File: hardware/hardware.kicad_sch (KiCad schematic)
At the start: 14 parts, among them J1 AVR-ISP-6, U1 AMS1117-3.3, U2 ATmega88PA-A, U3 CH340C, U4 MPU-6050, Y1 Crystal

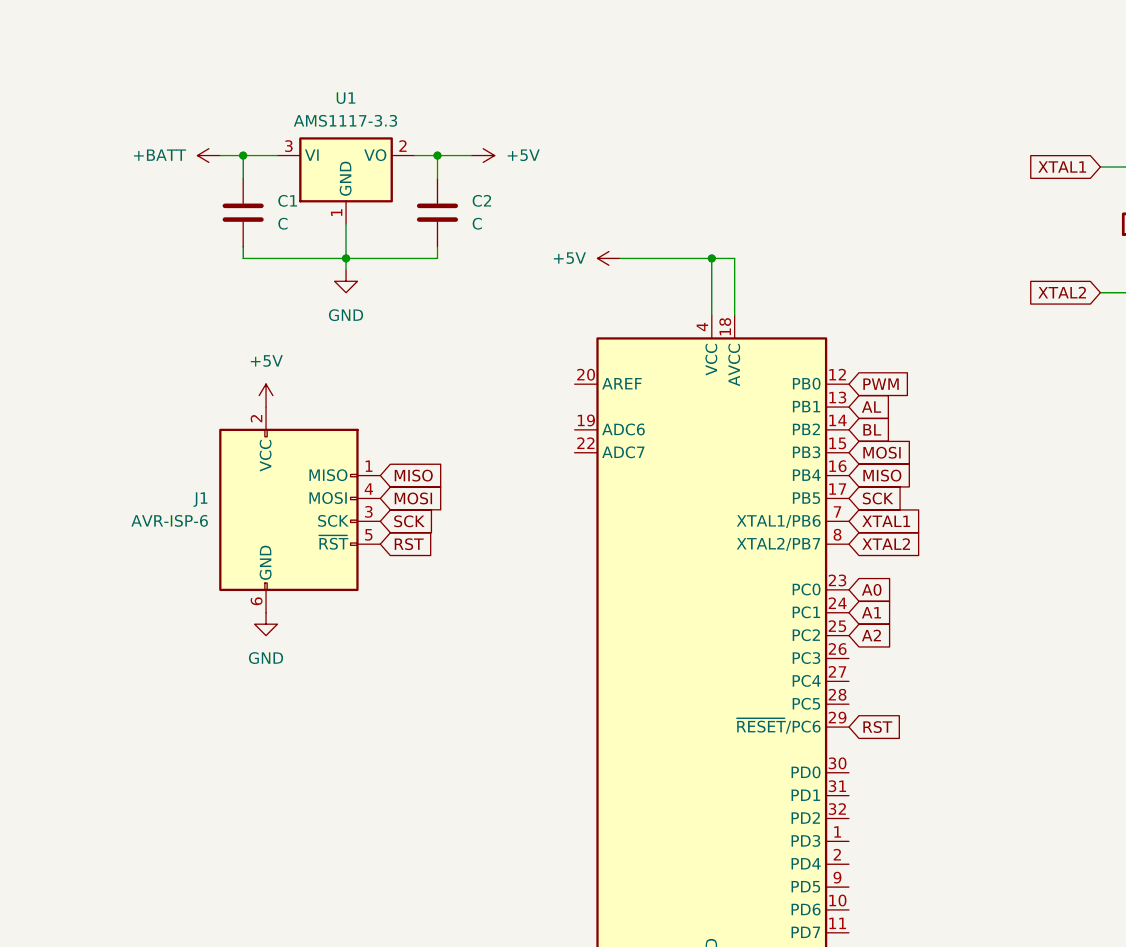
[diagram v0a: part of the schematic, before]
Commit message: up
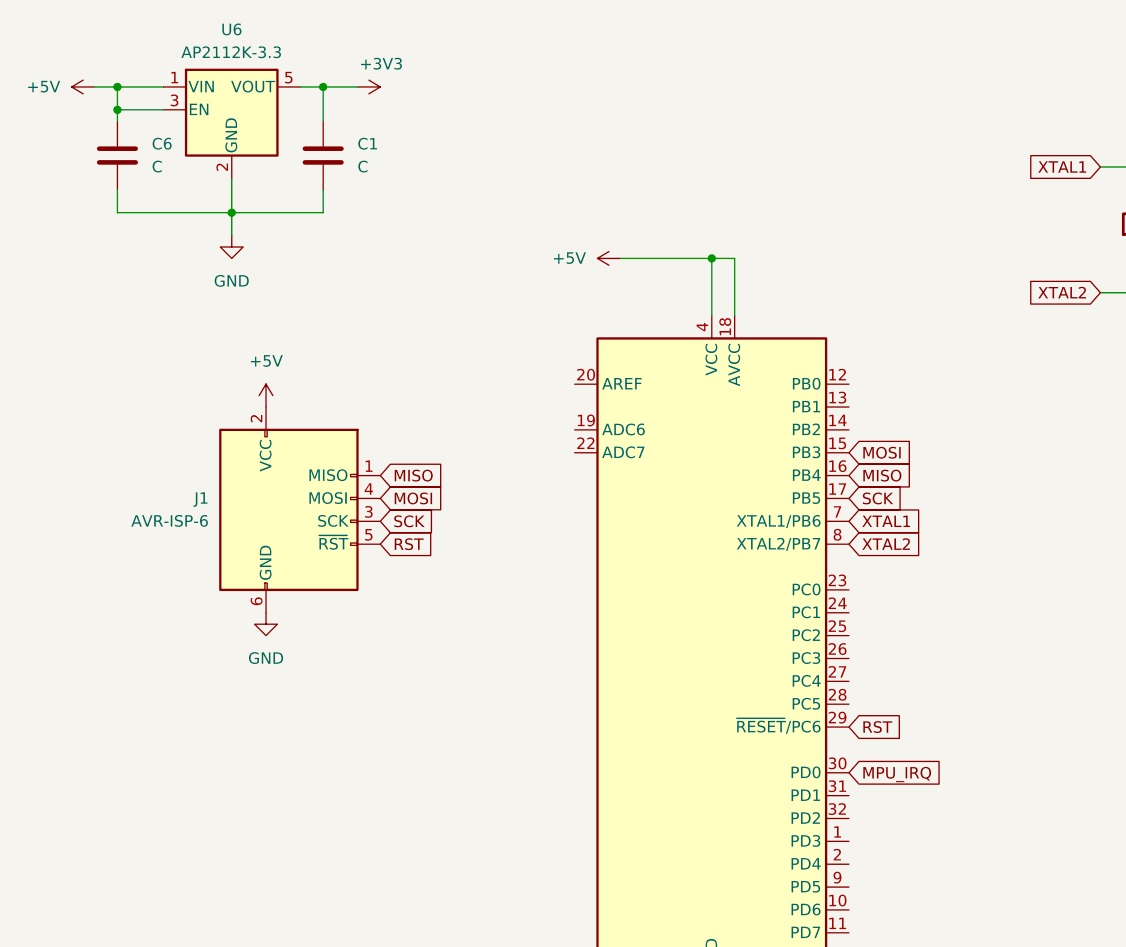
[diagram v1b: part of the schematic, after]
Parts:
- removed C2: C, Capacitor_SMD:C_0603_1608Metric, symbol Device:C
- removed U1: AMS1117-3.3, Package_TO_SOT_SMD:SOT-223-3_TabPin2, symbol Regulator_Linear:AMS1117-3.3
- added C6: C, Capacitor_SMD:C_0603_1608Metric, symbol Device:C
- added U6: AP2112K-3.3, Package_TO_SOT_SMD:SOT-23-5, symbol Regulator_Linear:AP2112K-3.3
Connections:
- net +BATT is gone; now on net +3V3: C1.1
- net +3V3: now also U6.5 (VOUT)
- net +5V: now also C6.1, U6.1 (VIN), U6.3 (EN)
- net GND: now also C6.2, U6.2 (GND)
- net MPU_IRQ: now also U2.30 (PD0)
- net A0: no longer names the net of U2.23 (PC0)
- net A1: no longer names the net of U2.24 (PC1)
- net A2: no longer names the net of U2.25 (PC2)
- net AL: no longer names the net of U2.13 (PB1)
- net BL: no longer names the net of U2.14 (PB2)
- net PWM: no longer names the net of U2.12 (PB0)

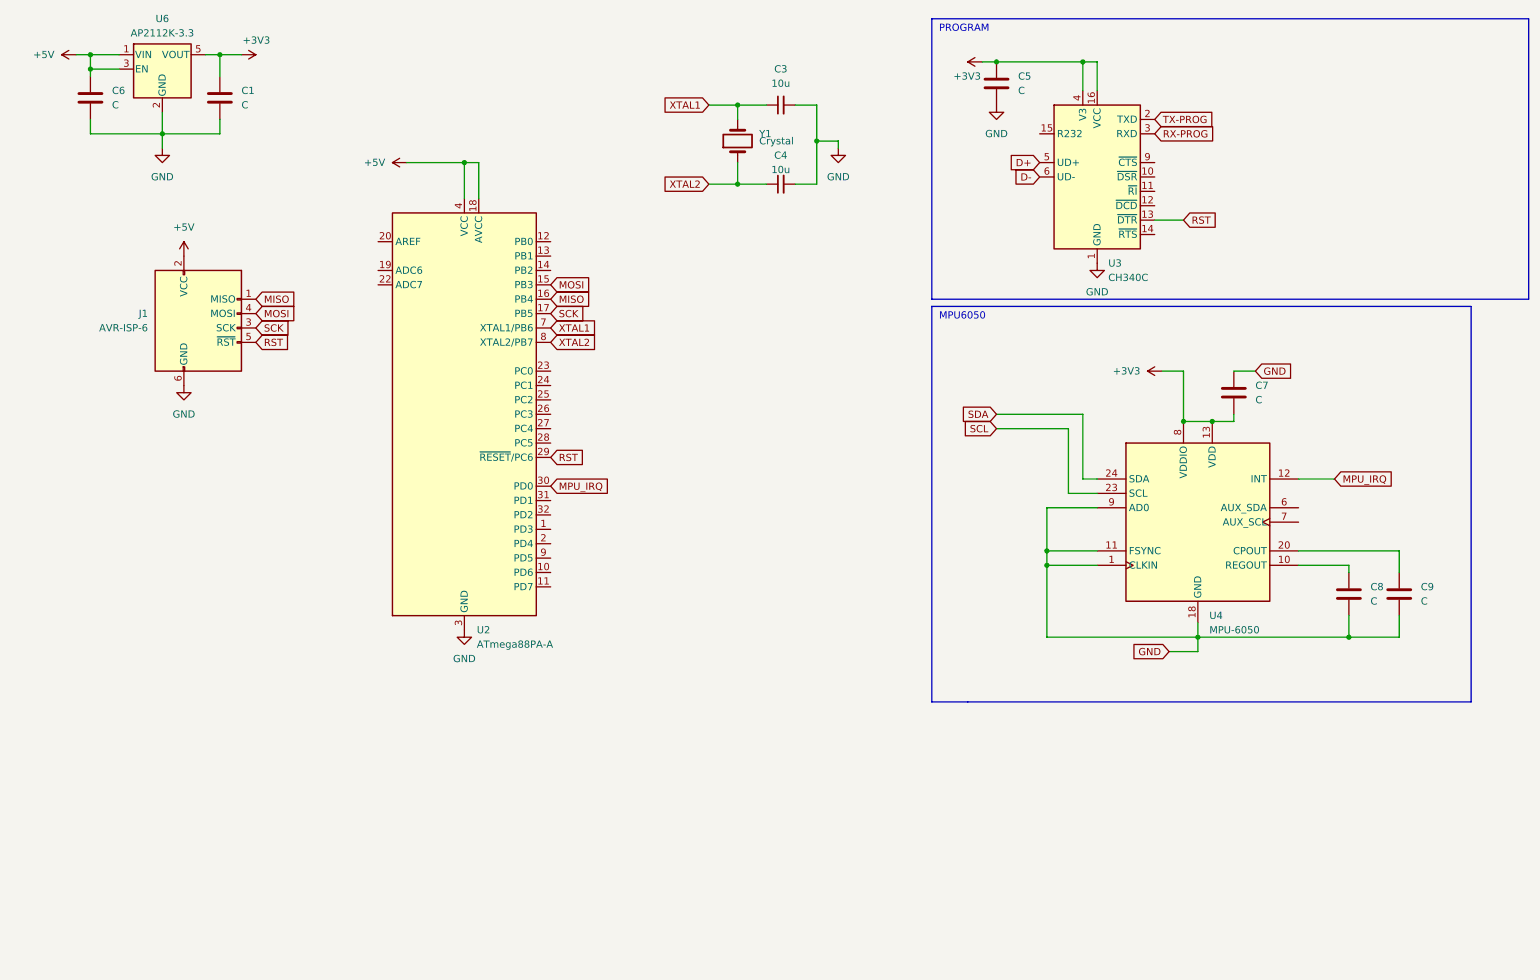
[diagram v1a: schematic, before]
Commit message: up
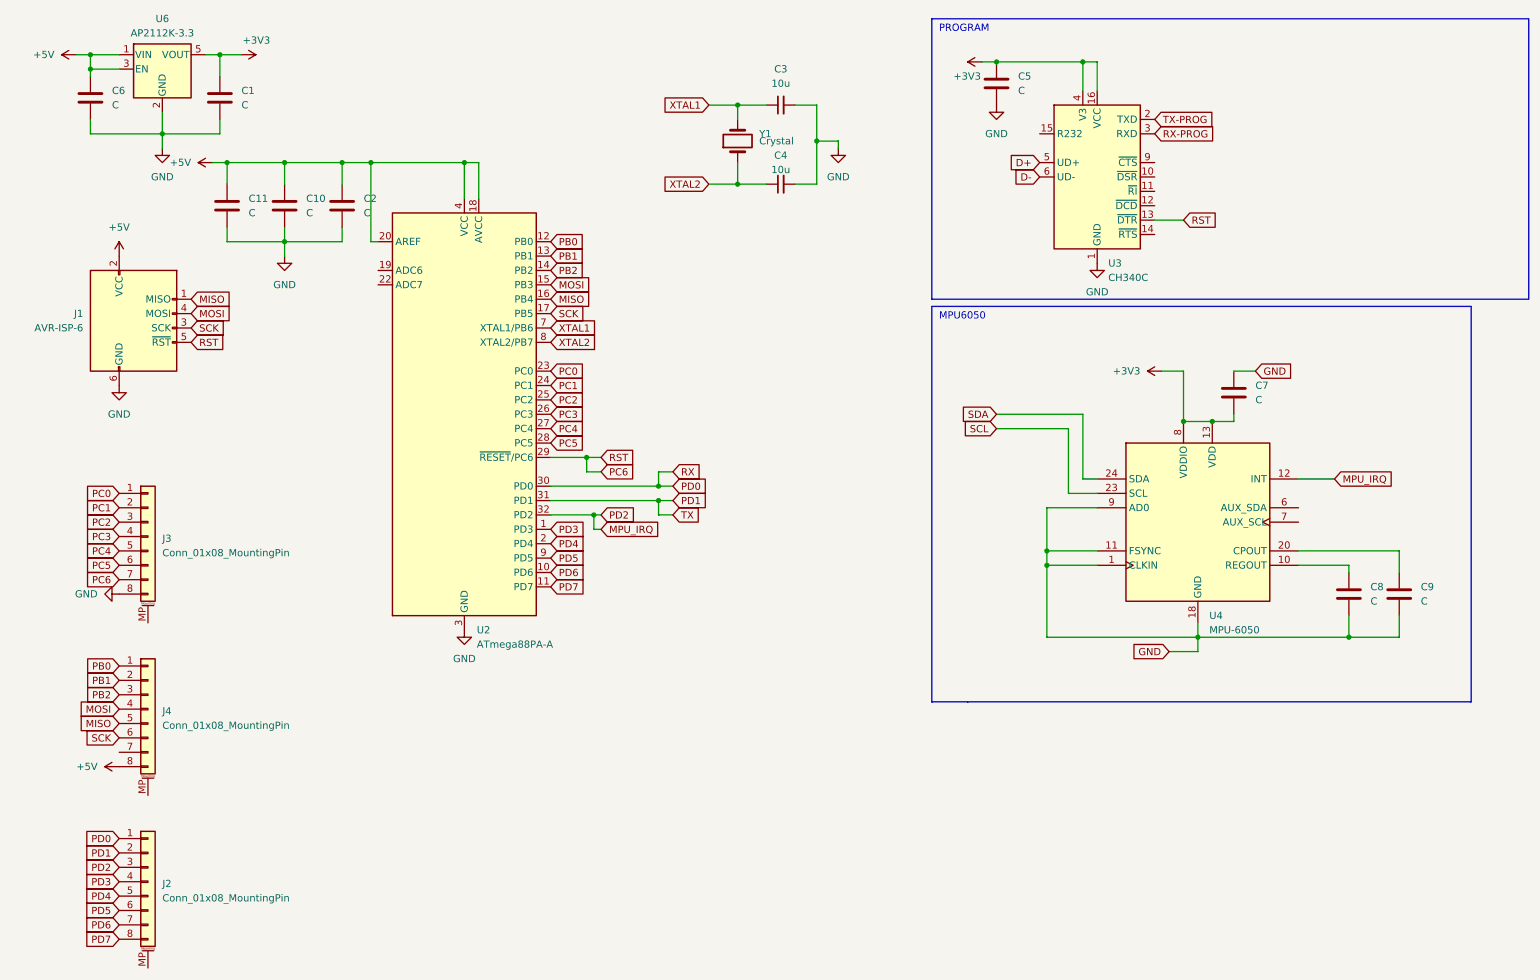
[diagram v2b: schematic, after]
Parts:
- added C10, C11, C2: C, Capacitor_SMD:C_0603_1608Metric, symbol Device:C
- added J2, J3, J4: Conn_01x08_MountingPin, Connector_PinHeader_2.54mm:PinHeader_1x08_P2.54mm_Vertical, symbol Connector_Generic_MountingPin:Conn_01x08_MountingPin
- Y1: footprint Crystal:Crystal_SMD_HC49-SD -> Crystal:Crystal_SMD_Abracon_ABM7-2Pin_6.0x3.5mm
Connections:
- net +5V: now also U2.20 (AREF), C10.1, C11.1, C2.1, J4.8 (Pin_8)
- net GND: now also C10.2, C11.2, C2.2, J3.8 (Pin_8)
- net MISO: now also J4.5 (Pin_5)
- net MOSI: now also J4.4 (Pin_4)
- net MPU_IRQ: now also U2.32 (PD2), J2.3 (Pin_3); no longer U2.30 (PD0)
- net SCK: now also J4.6 (Pin_6)
- net PD3: now reaches U2.1 (PD3)
- net PD3: now also J2.4 (Pin_4)
- net PD6: now reaches U2.10 (PD6)
- net PD6: now also J2.7 (Pin_7)
- net PD7: now reaches U2.11 (PD7)
- net PD7: now also J2.8 (Pin_8)
- net PB0: now reaches U2.12 (PB0)
- net PB0: now also J4.1 (Pin_1)
- net PB1: now reaches U2.13 (PB1)
- net PB1: now also J4.2 (Pin_2)
- net PB2: now reaches U2.14 (PB2)
- net PB2: now also J4.3 (Pin_3)
- net PD4: now reaches U2.2 (PD4)
- net PD4: now also J2.5 (Pin_5)
- net PC0: now reaches U2.23 (PC0)
- net PC0: now also J3.1 (Pin_1)
- net PC1: now reaches U2.24 (PC1)
- net PC1: now also J3.2 (Pin_2)
- net PC2: now reaches U2.25 (PC2)
- net PC2: now also J3.3 (Pin_3)
- net PC3: now reaches U2.26 (PC3)
- net PC3: now also J3.4 (Pin_4)
- net PC4: now reaches U2.27 (PC4)
- net PC4: now also J3.5 (Pin_5)
- net PC5: now reaches U2.28 (PC5)
- net PC5: now also J3.6 (Pin_6)
- net PD1: now reaches U2.31 (PD1)
- net PD1: now also J2.2 (Pin_2)
- net PD5: now reaches U2.9 (PD5)
- net PD5: now also J2.6 (Pin_6)
- net RST renamed PC6
- net PC6: now also J3.7 (Pin_7)
- new net PD0: J2.1 (Pin_1), U2.30 (PD0)
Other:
- moved on the sheet: J1

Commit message: up
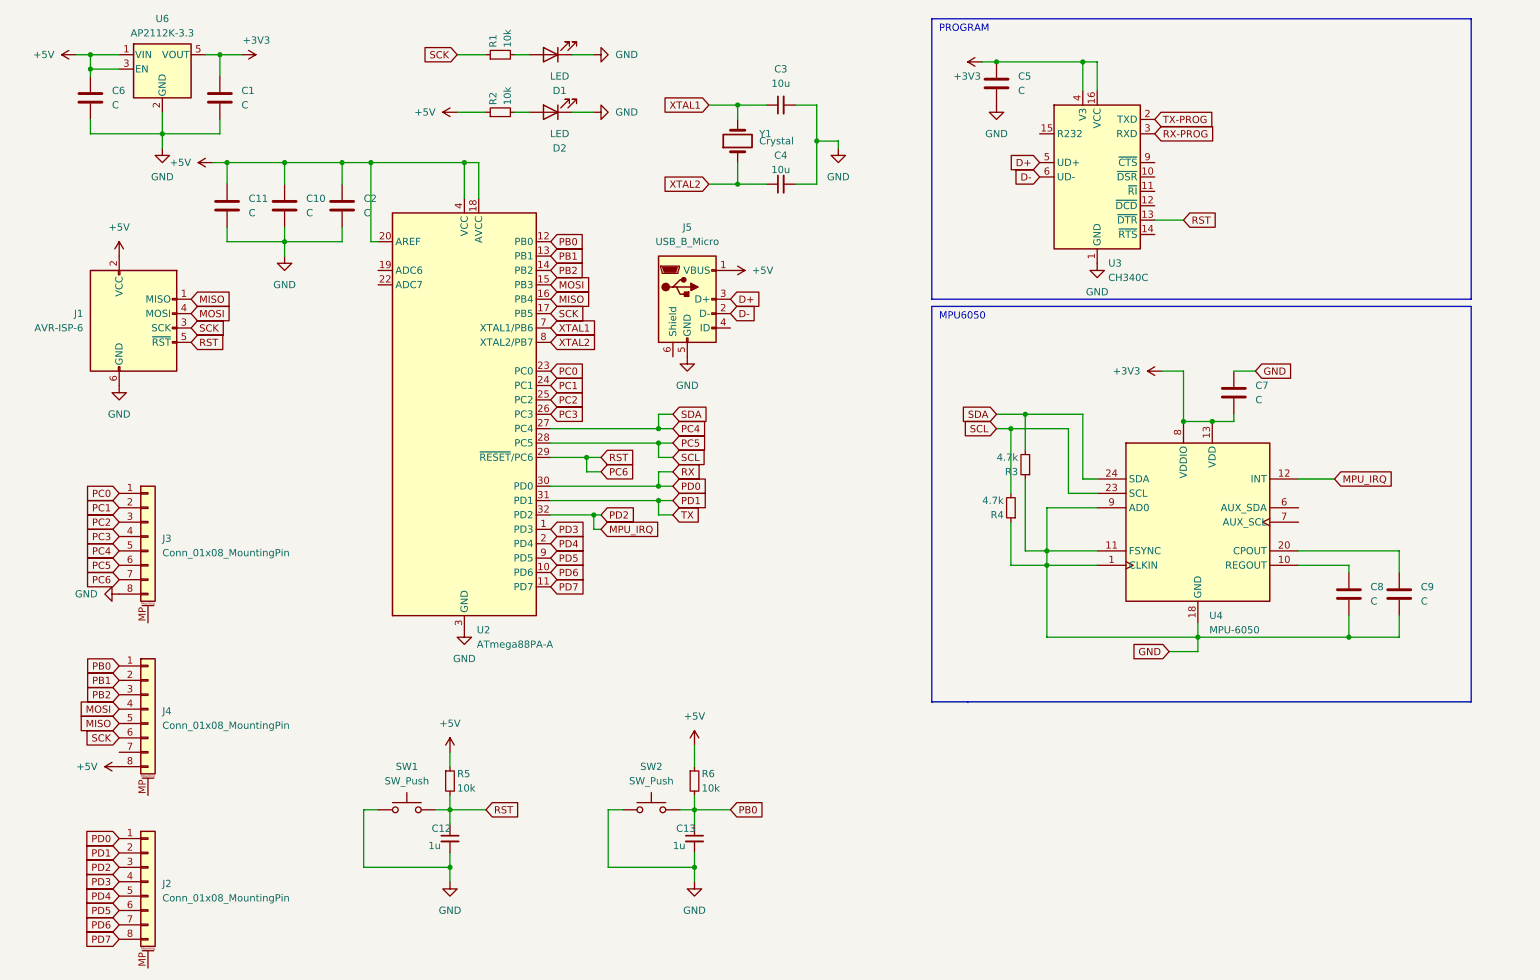
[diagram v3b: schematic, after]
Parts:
- added C12, C13: 1u, Capacitor_SMD:C_0603_1608Metric, symbol Device:C_Small
- added D1, D2: LED, Diode_SMD:D_0603_1608Metric, symbol Device:LED
- added J5: USB_B_Micro, Connector_USB:USB_Micro-B_GCT_USB3076-30-A, symbol Connector:USB_B_Micro
- added R1, R2, R5, R6: 10k, Resistor_SMD:R_0603_1608Metric, symbol Device:R_Small
- added R3, R4: 4.7k, Resistor_SMD:R_0603_1608Metric, symbol Device:R_Small
- added SW1, SW2: SW_Push, Button_Switch_SMD:SW_Push_SPST_NO_Alps_SKRK, symbol Switch:SW_Push
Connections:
- net SCL is gone; now on net PC5: U4.23 (SCL)
- net SDA is gone; now on net PC4: U4.24 (SDA)
- net +5V: now also J5.1 (VBUS), R2.1, R5.1, R6.1
- net D+: now also J5.3 (D+)
- net D-: now also J5.2 (D-)
- net GND: now also C12.2, C13.2, D1.1 (K), D2.1 (K), J5.5 (GND), R3.1, R4.1, SW1.1, SW2.1
- net PB0: now also C13.1, R6.2, SW2.2
- net PC4: now also R3.2
- net PC5: now also R4.2
- net PC6: now also C12.1, R5.2, SW1.2
- net SCK: now also R1.1
- new net: D2.2 (A), R2.2
- new net: D1.2 (A), R1.2
